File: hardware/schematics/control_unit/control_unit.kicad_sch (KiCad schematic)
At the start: 2 parts, among them J1 6P6C

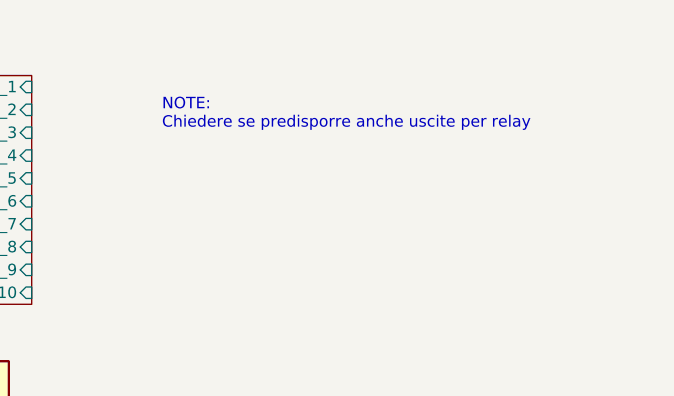
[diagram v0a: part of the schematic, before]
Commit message: chore
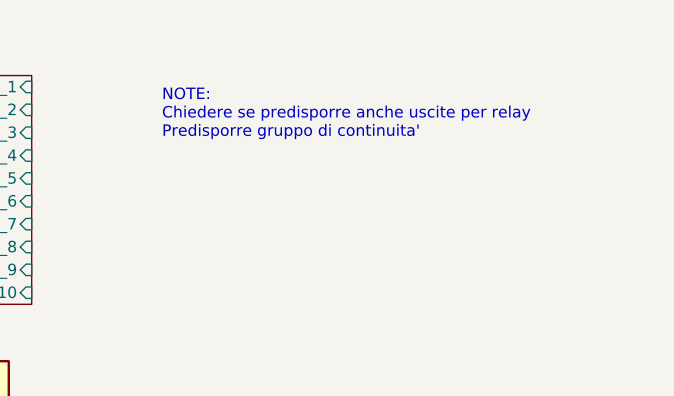
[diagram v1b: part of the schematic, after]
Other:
- note added: "NOTE: Chiedere se predisporre anche uscite per relay Predisporre gruppo di continuita'"
- note removed: "NOTE: Chiedere se predisporre anche uscite per relay"
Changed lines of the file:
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@@
 		)
 	)
-	(text "NOTE:\nChiedere se predisporre anche uscite per relay"
+	(text "NOTE:\nChiedere se predisporre anche uscite per relay\nPredisporre gruppo di continuita'"
 		(exclude_from_sim no)
 		(at 146.558 29.718 0)

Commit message: chore
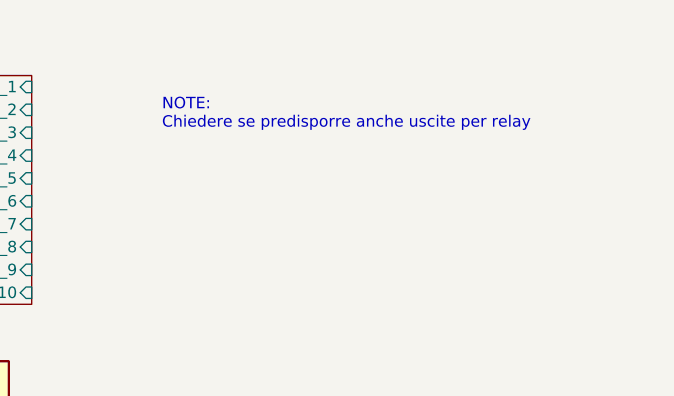
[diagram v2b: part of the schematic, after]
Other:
- note added: "NOTE: Chiedere se predisporre anche uscite per relay"
- note removed: "NOTE: Chiedere se predisporre anche uscite per relay Predisporre gruppo di continuita'"
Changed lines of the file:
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@@
 		)
 	)
-	(text "NOTE:\nChiedere se predisporre anche uscite per relay\nPredisporre gruppo di continuita'"
+	(text "NOTE:\nChiedere se predisporre anche uscite per relay"
 		(exclude_from_sim no)
 		(at 146.558 29.718 0)
@@
 		(dnp no)
 		(fields_autoplaced yes)
-		(property "Reference" "#PWR010"
+		(property "Reference" "#PWR011"
 			(at 121.92 29.21 0)
 			(effects
@@
 			(project "control_unit"
 				(path "/95f83be4-8e7e-4d00-b795-d60cd8e47b85"
-					(reference "#PWR010")
+					(reference "#PWR011")
 					(unit 1)
 				)
@@
 		(dnp no)
 		(fields_autoplaced yes)
-		(property "Reference" "#PWR011"
+		(property "Reference" "#PWR010"
 			(at 115.57 67.31 0)
 			(effects
@@
 			(project "control_unit"
 				(path "/95f83be4-8e7e-4d00-b795-d60cd8e47b85"
-					(reference "#PWR011")
+					(reference "#PWR010")
 					(unit 1)
 				)
@@
 		(dnp no)
 		(fields_autoplaced yes)
-		(property "Reference" "#PWR08"
+		(property "Reference" "#PWR07"
 			(at 92.71 58.42 0)
 			(effects
@@
 			(project "control_unit"
 				(path "/95f83be4-8e7e-4d00-b795-d60cd8e47b85"
-					(reference "#PWR08")
+					(reference "#PWR07")
 					(unit 1)
 				)
@@
 		(dnp no)
 		(fields_autoplaced yes)
-		(property "Reference" "#PWR012"
+		(property "Reference" "#PWR09"
 			(at 109.22 77.47 0)
 			(effects
@@
 			(project "control_unit"
 				(path "/95f83be4-8e7e-4d00-b795-d60cd8e47b85"
-					(reference "#PWR012")
+					(reference "#PWR09")
 					(unit 1)
 				)
@@
 		(dnp no)
 		(fields_autoplaced yes)
-		(property "Reference" "#PWR07"
+		(property "Reference" "#PWR06"
 			(at 82.55 86.36 0)
 			(effects
@@
 			(project "control_unit"
 				(path "/95f83be4-8e7e-4d00-b795-d60cd8e47b85"
-					(reference "#PWR07")
+					(reference "#PWR06")
 					(unit 1)
 				)
@@
 		(dnp no)
 		(fields_autoplaced yes)
-		(property "Reference" "#PWR06"
+		(property "Reference" "#PWR08"
 			(at 99.06 81.28 0)
 			(effects
@@
 			(project "control_unit"
 				(path "/95f83be4-8e7e-4d00-b795-d60cd8e47b85"
-					(reference "#PWR06")
+					(reference "#PWR08")
 					(unit 1)
 				)
@@
 		(dnp no)
 		(fields_autoplaced yes)
-		(property "Reference" "#PWR01"
+		(property "Reference" "#PWR02"
 			(at 31.75 40.64 0)
 			(effects
@@
 			(project "control_unit"
 				(path "/95f83be4-8e7e-4d00-b795-d60cd8e47b85"
-					(reference "#PWR01")
+					(reference "#PWR02")
 					(unit 1)
 				)
@@
 		(dnp no)
 		(fields_autoplaced yes)
-		(property "Reference" "#PWR09"
+		(property "Reference" "#PWR012"
 			(at 121.92 57.15 0)
 			(effects
@@
 			(project "control_unit"
 				(path "/95f83be4-8e7e-4d00-b795-d60cd8e47b85"
-					(reference "#PWR09")
+					(reference "#PWR012")
 					(unit 1)
 				)
@@
 		(dnp no)
 		(fields_autoplaced yes)
-		(property "Reference" "#PWR02"
+		(property "Reference" "#PWR01"
 			(at 29.21 26.67 0)
 			(effects
@@
 			(project "control_unit"
 				(path "/95f83be4-8e7e-4d00-b795-d60cd8e47b85"
-					(reference "#PWR02")
-					(unit 1)
-				)
+					(reference "#PWR01")
+					(unit 1)
+				)
